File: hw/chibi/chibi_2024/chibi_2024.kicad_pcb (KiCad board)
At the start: 2 copper layers, 100 x 78 mm, 114 parts, among them P1 VIN, P2 VIN, P3 GND, P4 CONN_02X05, P5 SWD, P6 GND, Q1 AO3415A, Q10 Q_NPN_CBE, Q11 Q_NPN_CBE, Q2 AO3415A, Q3 AO3415A, Q4 AO3415A, Q5 AO3415A, Q6 AO3415A, Q7 AO3415A, Q8 AO3415A, Q9 Q_PNP_CBE, SW1 USER, SW2 RESET, U1 LD1117S33CTR, U2 SP3485CN, U3 STM32F030F4Px, U4 LM358, U5 74HC595_mine, U6 LM393, U7 74HC595_mine, U8 MBI5026, U9 MBI5026, Y1 8MHz

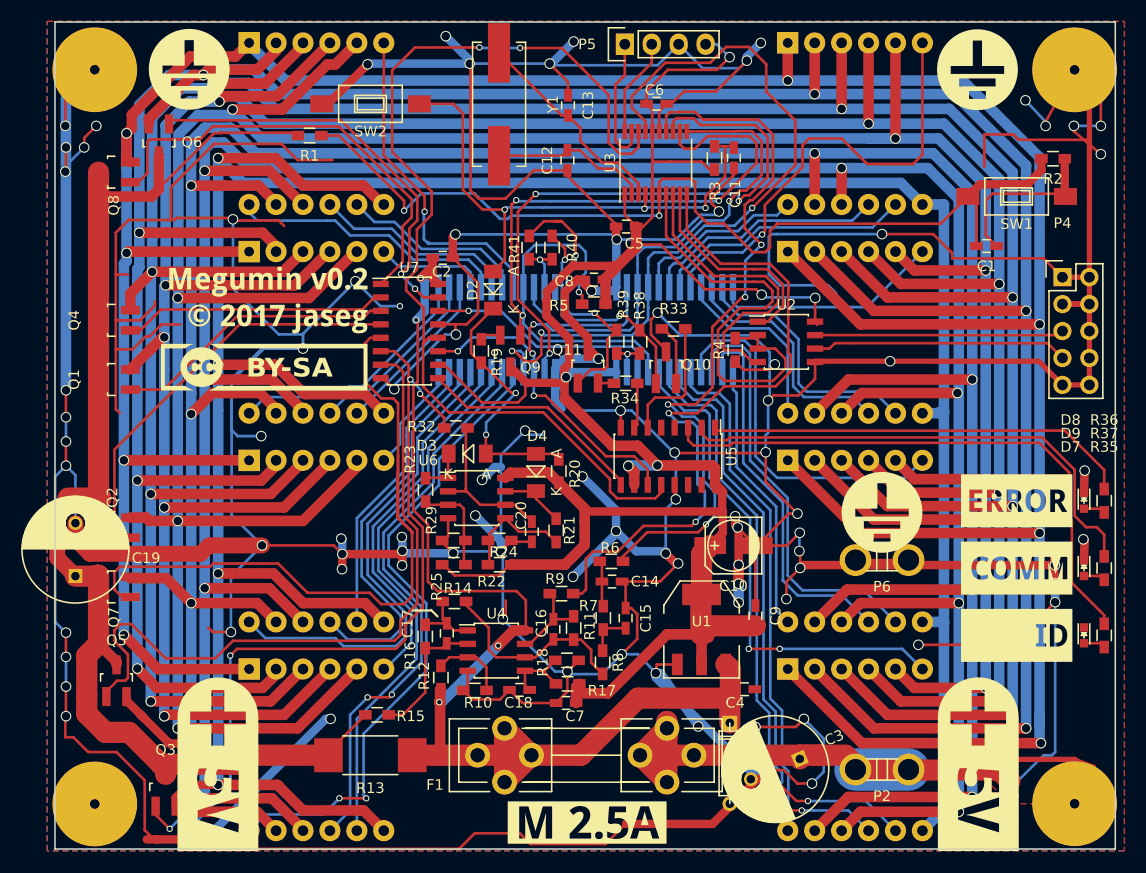
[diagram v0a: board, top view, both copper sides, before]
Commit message: Second board revision
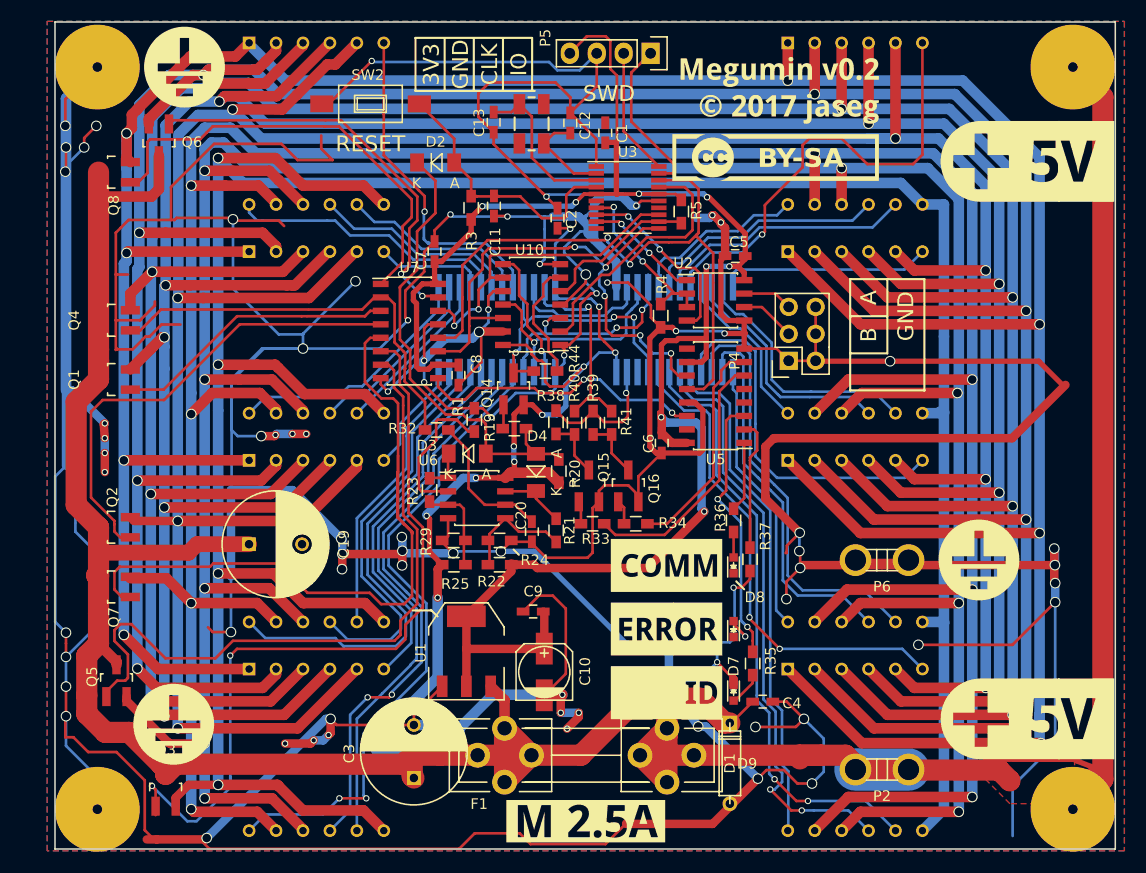
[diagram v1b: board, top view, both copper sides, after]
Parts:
- removed C14, C15: 220n, Capacitors_SMD:C_0603_HandSoldering
- removed C16, C17: comp, Capacitors_SMD:C_0603_HandSoldering
- removed C18: 100n, Capacitors_SMD:C_0603_HandSoldering
- removed Q10, Q11: Q_NPN_CBE, TO_SOT_Packages_SMD:SOT-23_Handsoldering
- removed Q9: Q_PNP_CBE, TO_SOT_Packages_SMD:SOT-23_Handsoldering
- removed R10, R16: 47k, Resistors_SMD:R_0603_HandSoldering
- removed R11: 100k, Resistors_SMD:R_0603_HandSoldering
- removed R12, R14, R15, R2: 10k, Resistors_SMD:R_0603_HandSoldering
- removed R13: 0.1, Resistors_SMD:R_2512_HandSoldering
- removed R17, R18, R6, R7, R8: 4k7, Resistors_SMD:R_0603_HandSoldering
- removed R9: 1k, Resistors_SMD:R_0603_HandSoldering
- removed REF** (x2): m3_pillar, footprints:m3_pillar
- removed SW1: USER, Buttons_Switches_SMD:SW_SPST_FSMSM
- removed U4: LM358, Housings_SOIC:SOIC-8_3.9x4.9mm_Pitch1.27mm
- removed the svg2mod at (61.7, 48.2)
- removed the svg2mod at (64.4, 113.8)
- removed the svg2mod at (127.0, 90.0)
- removed the svg2mod at (136.1, 113.7)
- removed the svg2mod at (136.0, 48.2)
- added P1: VIN, footprints:m3_pillar, F.Cu at (159.3, 115.3)
- added P3: GND, footprints:m3_pillar, F.Cu at (52.5, 117.4)
- added Q14: Q_PNP_BEC, TO_SOT_Packages_SMD:SOT-23_Handsoldering, F.Cu at (92.2, 78.3)
- added Q15: Q_NPN_BEC, TO_SOT_Packages_SMD:SOT-23_Handsoldering, F.Cu at (99.3, 87.5)
- added Q16: Q_NPN_BEC, TO_SOT_Packages_SMD:SOT-23_Handsoldering, F.Cu at (103.1, 87.5)
- added R44: 1k, Resistors_SMD:R_0603_HandSoldering, F.Cu at (95.2, 76.7)
- added U10: 74HCT125, Housings_SOIC:SOIC-14_3.9x8.7mm_Pitch1.27mm, F.Cu at (94.0, 70.4)
- added svg2mod: G***, footprints:label_plus_04, F.Cu at (140.7, 56.9)
- added svg2mod: G***, footprints:label_gnd_04, F.Cu at (60.2, 110.0)
- added svg2mod: G***, footprints:label_plus_04, F.Cu at (140.7, 109.5)
- added svg2mod: G***, footprints:label_gnd_04, F.Cu at (136.1, 94.5)
- added svg2mod: G***, footprints:label_gnd_04, F.Cu at (61.2, 48.0)
- P4: value CONN_02X05 -> CONN_02X03; footprint Pin_Headers:Pin_Header_Straight_2x05 -> Socket_Strips:Socket_Strip_Straight_2x03
- R1: value 10k -> 47k
- Y1: value 8MHz -> 25M; footprint Crystals:Crystal_HC49-SD_SMD -> footprints:CRYSTAL-SMD-5X3
- moved P3 92.3 mm to (52.9, 47.8)
- moved svg2mod 52.1 mm to (115.6, 52.7)
- moved C7 44.3 mm to (84.8, 65.4), turned to 270 degrees
- moved C1 37.5 mm to (100.9, 54.2), turned to 270 degrees
- moved C3 36.4 mm to (82.8, 115.0), turned to 90 degrees
- moved svg2mod 35.2 mm to (106.7, 101.0)
- moved R36 35.0 mm to (113.0, 90.8)
- moved D8 33.6 mm to (113.0, 95.0), turned to 90 degrees
- moved D9 33.5 mm to (113.0, 101.0), turned to 90 degrees
- moved D7 33.5 mm to (113.0, 107.0)
- moved svg2mod 33.5 mm to (106.7, 107.0)
- moved R37 33.4 mm to (114.5, 94.4)
- moved R35 33.3 mm to (114.8, 104.2)
- moved svg2mod 33.0 mm to (106.7, 95.0)
- moved C6 32.0 mm to (106.2, 83.5), turned to 90 degrees
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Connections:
- net /MOSI_C1 renamed /MOSI_C1_HV
- C1 pad 1: Net-(C1-Pad1) -> GND
- C1 pad 2: /USER_BTN -> +3V3
- C19 pad 1: /SEG_COM_MEAS -> VDD
- C20 pad 1: /WD_COMP -> /WD_COMP1
- C3 pad 1: /VDD_PRE_FUSE -> VDD
- P4 pad 3: GND -> /RS485_A
- Q1 pad 1: /SEG_A_CTRL -> /SEG_C_CTRL
- Q1 pad 3: /SEG_COM_MEAS -> VDD
- Q2 pad 1: /SEG_E_CTRL -> /SEG_G_CTLR
- Q2 pad 3: /SEG_COM_MEAS -> VDD
- Q3 pad 1: /SEG_A_CTRL -> /SEG_B_CTRL
- Q3 pad 3: /SEG_COM_MEAS -> VDD
- Q4 pad 1: /SEG_A_CTRL -> /SEG_DP_CTRL
- Q4 pad 3: /SEG_COM_MEAS -> VDD
- Q5 pad 1: /SEG_E_CTRL -> /SEG_F_CTRL
- Q5 pad 3: /SEG_COM_MEAS -> VDD
- Q6 pad 1: /SEG_A_CTRL -> /SEG_D_CTRL
- Q6 pad 3: /SEG_COM_MEAS -> VDD
- Q7 pad 3: /SEG_COM_MEAS -> VDD
- Q8 pad 3: /SEG_COM_MEAS -> VDD
- R1 pad 1: /USER_BTN -> GND
- R1 pad 2: /SEG_COM_MEAS -> Net-(R1-Pad2)
- R20 pad 1: +3V3 -> VDD
- R25 pad 2: +3V3 -> VDD
- R32 pad 1: /WD_COMP -> /WD_COMP1
- R32 pad 2: /SEG_A_CTRL -> /SEG_DP_CTRL
- U3 pad 1: +3V3 -> GND
- U3 pad 10: /CMEAS_OUT -> Net-(U3-Pad10)
- U3 pad 14: /CMEAS_OFFX_COMP -> Net-(U3-Pad14)
- U3 pad 6: /USER_BTN -> Net-(U3-Pad6)
- U5 pad 9: /MOSI_C3 -> Net-(U5-Pad9)
- U6 pad 2: /WD_COMP -> Net-(R1-Pad2)
- U6 pad 6: /WD_COMP -> /WD_COMP1
- U6 pad 8: +3V3 -> VDD
- U7 pad 14: /MOSI_C2 -> /MOSI_C0
- U7 pad 15: /SEG_A_CTRL -> /SEG_D_CTRL
- U7 pad 16: VDD -> +3V3
- U7 pad 2: /SEG_A_CTRL -> /SEG_DP_CTRL
- U7 pad 3: /SEG_A_CTRL -> /SEG_C_CTRL
- U7 pad 4: /SEG_E_CTRL -> /SEG_G_CTLR
- U7 pad 6: /SEG_A_CTRL -> /SEG_B_CTRL
- U7 pad 7: /SEG_E_CTRL -> /SEG_F_CTRL
- U7 pad 9: /MOSI_C3 -> Net-(U5-Pad14)
- U8 pad 21: /~OE -> /~OE_HV_CB
- U8 pad 22: /MOSI_C2 -> /mux_mod_right/SDO
- U8 pad 24: +3V3 -> VDD
- U8 pad 3: /SCK -> /SCK_HV
- U8 pad 4: /STROBE -> /STROBE_HV
- U9 pad 2: /MOSI_C0 -> /MOSI_C0_HV
- U9 pad 21: /~OE -> /~OE_HV_CB
- U9 pad 24: /mux_mod_left/VDD -> VDD
- U9 pad 3: /SCK -> /SCK_HV
- U9 pad 4: /STROBE -> /STROBE_HV
- Y1 pad 1: /XT2 -> /XT1
- Y1 pad 2: /XT1 -> (no net)
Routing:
- net /SEG_A_CTRL: track 238.5 -> 70.0 mm, vias 6 -> 0
- net VDD: track 117.4 -> 282.8 mm, vias 4 -> 10
- net /SEG_COM_MEAS: track 136.7 -> 0.00 mm
- net /SEG_E_CTRL: track 147.4 -> 42.5 mm
- net /USER_BTN: track 92.1 -> 0.00 mm, vias 2 -> 0
- net /VDD_PRE_FUSE: track 84.4 -> 159.3 mm
- net /SEG_B_CTRL: track 0.00 -> 74.6 mm, vias 0 -> 2
- net /CMEAS_OFFX_COMP: track 69.6 -> 0.00 mm, vias 4 -> 0
- net /~OE: track 82.5 -> 14.9 mm, vias 4 -> 0
- net /CMEAS_OUT: track 65.9 -> 0.00 mm, vias 2 -> 0
- net /SEG_F_CTRL: track 0.00 -> 65.5 mm
- net GND: track 1062.5 -> 1011.3 mm, vias 91 -> 78
- net /STROBE: track 74.6 -> 24.4 mm, vias 3 -> 0
- net /SEG_G_CTLR: track 0.00 -> 44.7 mm
- net /SEG_D_CTRL: track 0.00 -> 39.0 mm, vias 0 -> 2
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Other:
- net class Default: clearance 0.2 -> 0.16
- net class fuck_kicad: clearance 0.2 -> 0.16
- net class moar_pwr: clearance 0.2 -> 0.16
- rule trace_clearance: 0.2 -> 0.16
- board text added: "3V3"
- board text added: "A"
- board text added: "B"
- board text added: "CLK"
- board text added: "GND"
- board text added: "IO"
- board text added: "RESET"
- board text added: "SWD"

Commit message: Final silk art positioning
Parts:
- moved svg2mod 4.44 mm to (98.0, 78.5), turned to 0 degrees
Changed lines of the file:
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@@
     (links 279)
     (no_connects 0)
-    (area 47.31886 39.765768 160.611476 125.705685)
+    (area 44.876376 39.765768 160.611476 125.705685)
     (thickness 1.6)
     (drawings 33)
@@
   (page A4)
   (layers
-    (0 F.Cu signal)
-    (31 B.Cu signal hide)
+    (0 F.Cu signal hide)
+    (31 B.Cu signal)
     (32 B.Adhes user hide)
     (33 F.Adhes user hide)
     (34 B.Paste user hide)
     (35 F.Paste user hide)
-    (36 B.SilkS user hide)
-    (37 F.SilkS user)
-    (38 B.Mask user hide)
-    (39 F.Mask user)
+    (36 B.SilkS user)
+    (37 F.SilkS user hide)
+    (38 B.Mask user)
+    (39 F.Mask user hide)
     (40 Dwgs.User user hide)
     (41 Cmts.User user hide)
@@
   )
   (setup
-    (last_trace_width 2)
+    (last_trace_width 0.25)
     (user_trace_width 0.254)
     (user_trace_width 0.35)
@@
     (pad_to_mask_clearance 0.2)
     (aux_axis_origin 0 0)
-    (visible_elements FFFEFB7F)
+    (visible_elements FFFEFD7F)
     (pcbplotparams
       (layerselection 0x010fc_80000001)
@@
     (pad 2 smd rect (at 1.84912 1.14808 90) (size 1.89992 1.09982) (layers F.Cu F.Paste F.Mask))
   )
-  (module footprints:megumin locked (layer B.Cu)
-    (at 99.822 82.55 180)
+  (module footprints:megumin (layer B.Cu)
+    (at 98.044 78.486)
     (descr "Imported from megumin_kicad.svg")
     (tags svg2mod)
     (attr smd)
-    (fp_text reference svg2mod (at 0 36.065404 180) (layer B.SilkS) hide
+    (fp_text reference svg2mod (at 0 36.065404) (layer B.SilkS) hide
       (effects (font (thickness 0.3048)) (justify mirror))
     )
-    (fp_text value G*** (at 0 -36.065404 180) (layer B.SilkS) hide
+    (fp_text value G*** (at 0 -36.065404) (layer B.SilkS) hide
       (effects (font (thickness 0.3048)) (justify mirror))
     )
